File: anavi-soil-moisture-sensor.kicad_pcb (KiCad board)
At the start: 2 copper layers, 22.9 x 61 mm, 9 parts, among them P1 CONN_01X03, P2 CONN_01X01, P3 CONN_01X01, Q1 BC817

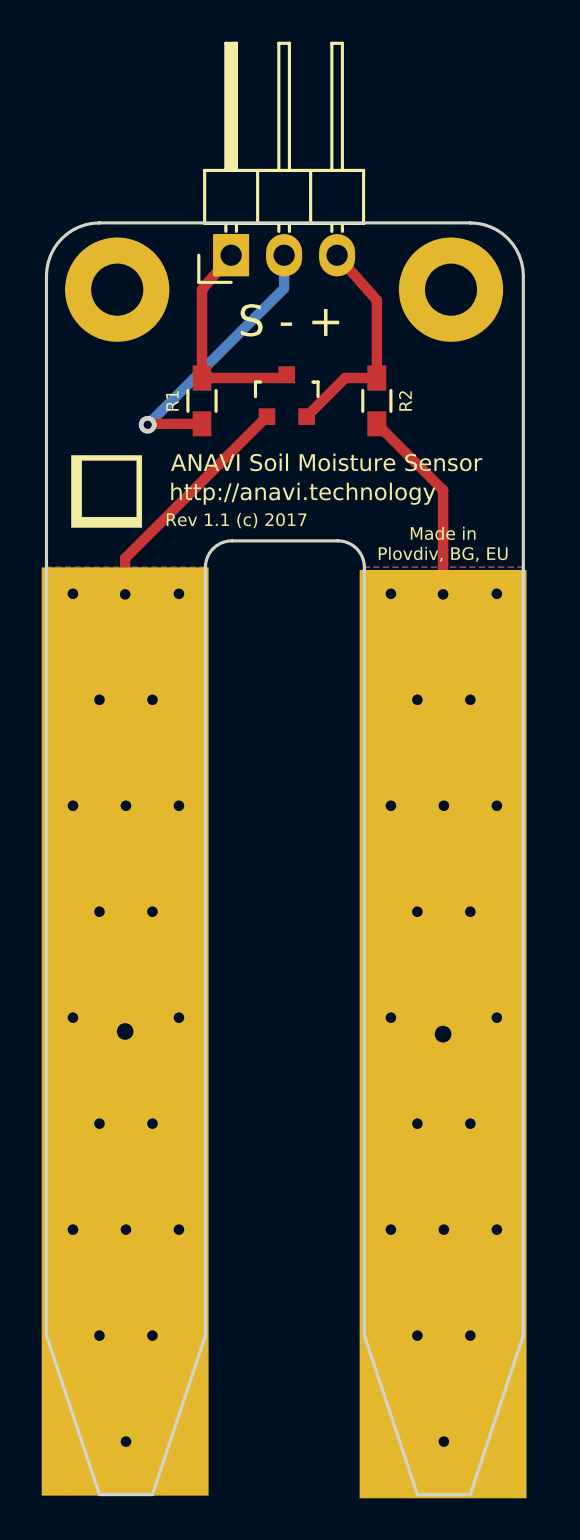
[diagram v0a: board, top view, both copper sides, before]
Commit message: anavi-soil-moisture-sensor.kicad_pcb: Revision 1.1
Signed-off-by: Leon Anavi <leon@anavi.org>
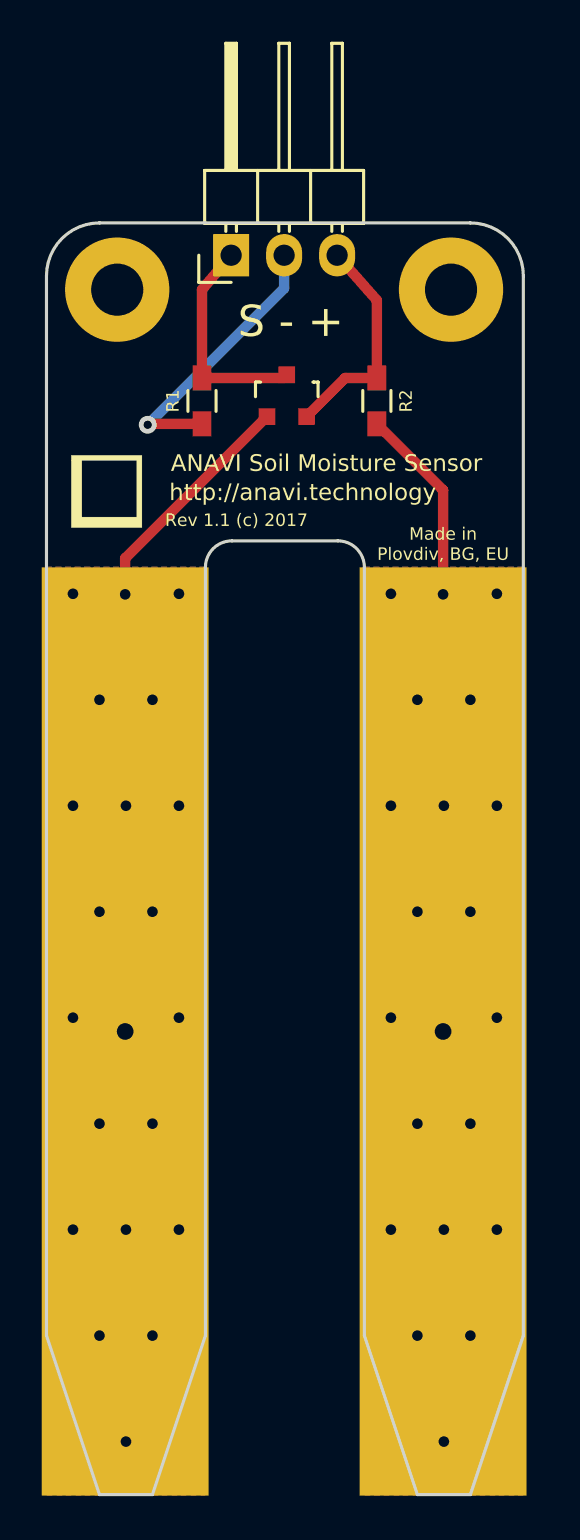
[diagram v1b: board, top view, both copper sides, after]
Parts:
- moved P3 0.13 mm to (156.1, 113.3)
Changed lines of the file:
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@@
     (links 7)
     (no_connects 0)
-    (area 136.996099 74.448599 160.006101 135.558601)
+    (area 130.493714 65.143999 166.432286 135.788)
     (thickness 1.6)
     (drawings 45)
@@
       (drillshape 0)
       (scaleselection 1)
-      (outputdirectory plots/plot-1.0/))
+      (outputdirectory plots/plot-1.1/))
   )
   (net 0 "")
@@
   )
   (module Wire_Pads:SolderWirePad_single_0-8mmDrill (layer Top)
-    (at 156.083 113.411)
+    (at 156.083 113.284)
     (fp_text reference P3 (at 0 -2.54) (layer F.SilkS) hide
       (effects (font (size 1 1) (thickness 0.15)))
